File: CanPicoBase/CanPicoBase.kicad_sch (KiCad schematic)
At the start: 17 parts, among them J1 3.50 CBUS, J2 5V select, J3 Grove 2mm, J4 Conn_01x20_Male, J5 Conn_01x20_Male, Q1 DMG2305UX-7, U1 AMS1117-5.0, U2 AMS1117-3.3, U3 Pico

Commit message: 20:38 Arrakis.local
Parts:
- J4, J5: footprint Connector_PinHeader_2.54mm:PinHeader_1x20_P2.54mm_Vertical -> Connector_PinSocket_2.54mm:PinSocket_1x20_P2.54mm_Vertical
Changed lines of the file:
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@@
     (property "Reference" "J4" (id 0) (at 191.135 34.29 0))
     (property "Value" "Conn_01x20_Male" (id 1) (at 191.135 36.83 0))
-    (property "Footprint" "Connector_PinHeader_2.54mm:PinHeader_1x20_P2.54mm_Vertical" (id 2) (at 190.5 62.23 0)
+    (property "Footprint" "Connector_PinSocket_2.54mm:PinSocket_1x20_P2.54mm_Vertical" (id 2) (at 190.5 62.23 0)
       (effects (font (size 1.27 1.27)) hide)
     )
@@
       (effects (font (size 1.27 1.27)) (justify right))
     )
-    (property "Footprint" "Connector_PinHeader_2.54mm:PinHeader_1x20_P2.54mm_Vertical" (id 2) (at 273.05 64.77 0)
+    (property "Footprint" "Connector_PinSocket_2.54mm:PinSocket_1x20_P2.54mm_Vertical" (id 2) (at 273.05 64.77 0)
       (effects (font (size 1.27 1.27)) hide)
     )
@@
     )
     (path "/1a850953-e696-40b6-a1fc-7a92a62063d4"
-      (reference "J4") (unit 1) (value "Conn_01x20_Male") (footprint "Connector_PinHeader_2.54mm:PinHeader_1x20_P2.54mm_Vertical")
+      (reference "J4") (unit 1) (value "Conn_01x20_Male") (footprint "Connector_PinSocket_2.54mm:PinSocket_1x20_P2.54mm_Vertical")
     )
     (path "/508c1793-b3ac-4a28-93d9-e73559a97305"
-      (reference "J5") (unit 1) (value "Conn_01x20_Male") (footprint "Connector_PinHeader_2.54mm:PinHeader_1x20_P2.54mm_Vertical")
+      (reference "J5") (unit 1) (value "Conn_01x20_Male") (footprint "Connector_PinSocket_2.54mm:PinSocket_1x20_P2.54mm_Vertical")
     )
     (path "/37118974-3a56-4fcc-9031-fa4d14c74939"

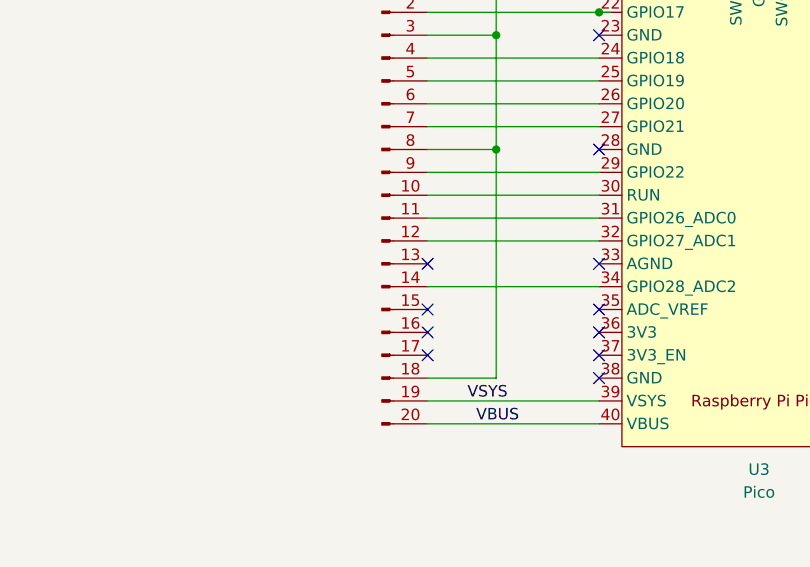
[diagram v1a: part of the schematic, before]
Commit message: 21:37 Titan.local
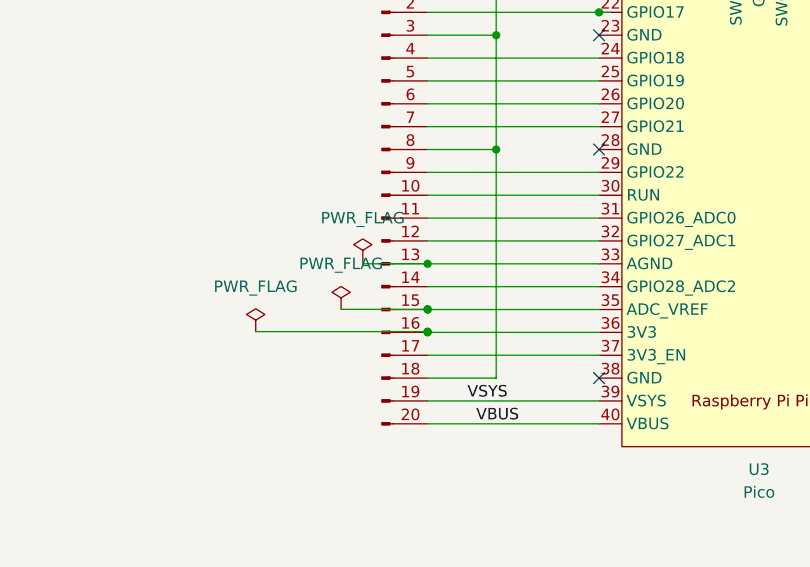
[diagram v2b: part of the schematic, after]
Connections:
- net at J4.13 (Pin_13): now also U3.33 (AGND)
- net at J4.15 (Pin_15): now also U3.35 (ADC_VREF)
- net at J4.16 (Pin_16): now also U3.36 (3V3)
- net at J4.17 (Pin_17): now also U3.37 (3V3_EN)
- no-connect marks 19 -> 11
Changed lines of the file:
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@@
   (junction (at 267.97 82.55) (diameter 0) (color 0 0 0 0)
   )
+  (junction (at 195.58 77.3836) (diameter 0) (color 0 0 0 0)
+  )
   (junction (at 34.065 120.5719) (diameter 0) (color 0 0 0 0)
   )
+  (junction (at 195.58 74.9115) (diameter 0) (color 0 0 0 0)
+  )
   (junction (at 58.42 62.1444) (diameter 0) (color 0 0 0 0)
   )
@@
   (junction (at 214.63 41.91) (diameter 0) (color 0 0 0 0)
   )
+  (junction (at 195.58 74.93) (diameter 0) (color 0 0 0 0)
+  )
   (junction (at 257.81 57.15) (diameter 0) (color 0 0 0 0)
   )
@@
   (junction (at 57.15 100.2425) (diameter 0) (color 0 0 0 0)
   )
+  (junction (at 195.58 77.47) (diameter 0) (color 0 0 0 0)
+  )
   (junction (at 203.2 44.45) (diameter 0) (color 0 0 0 0)
   )
+  (junction (at 195.58 69.85) (diameter 0) (color 0 0 0 0)
+  )
   (no_connect (at 250.19 69.85))
-  (no_connect (at 214.63 80.01))
-  (no_connect (at 195.58 69.85))
   (no_connect (at 214.63 82.55))
-  (no_connect (at 195.58 80.01))
   (no_connect (at 234.95 34.29))
   (no_connect (at 250.19 57.15))
@@
   (no_connect (at 22.86 29.21))
   (no_connect (at 229.87 34.29))
-  (no_connect (at 214.63 77.47))
-  (no_connect (at 195.58 74.93))
-  (no_connect (at 214.63 69.85))
   (no_connect (at 214.63 44.45))
-  (no_connect (at 214.63 74.93))
-  (no_connect (at 195.58 77.47))
   (no_connect (at 214.63 57.15))
   (wire (pts (xy 250.19 82.55) (xy 257.81 82.55))
@@
     (stroke (width 0) (type default) (color 0 0 0 0))
   )
+  (wire (pts (xy 188.379 69.85) (xy 195.58 69.85))
+    (stroke (width 0) (type default) (color 0 0 0 0))
+  )
   (wire (pts (xy 58.42 48.26) (xy 58.42 52.07))
     (stroke (width 0) (type default) (color 0 0 0 0))
@@
     (stroke (width 0) (type default) (color 0 0 0 0))
   )
+  (wire (pts (xy 195.58 77.3836) (xy 195.58 77.47))
+    (stroke (width 0) (type default) (color 0 0 0 0))
+  )
   (wire (pts (xy 250.19 41.91) (xy 267.97 41.91))
     (stroke (width 0) (type default) (color 0 0 0 0))
@@
     (stroke (width 0) (type default) (color 0 0 0 0))
   )
+  (wire (pts (xy 185.9652 74.9115) (xy 195.58 74.9115))
+    (stroke (width 0) (type default) (color 0 0 0 0))
+  )
   (wire (pts (xy 203.2 44.45) (xy 203.2 57.15))
     (stroke (width 0) (type default) (color 0 0 0 0))
@@
     (stroke (width 0) (type default) (color 0 0 0 0))
   )
+  (wire (pts (xy 195.58 74.93) (xy 214.63 74.93))
+    (stroke (width 0) (type default) (color 0 0 0 0))
+  )
   (wire (pts (xy 83.82 33.02) (xy 83.82 48.26))
     (stroke (width 0) (type default) (color 0 0 0 0))
@@
     (stroke (width 0) (type default) (color 0 0 0 0))
   )
+  (wire (pts (xy 176.4825 77.3828) (xy 195.58 77.3836))
+    (stroke (width 0) (type default) (color 0 0 0 0))
+  )
   (wire (pts (xy 29.21 120.65) (xy 34.065 120.65))
     (stroke (width 0) (type default) (color 0 0 0 0))
@@
     (stroke (width 0) (type default) (color 0 0 0 0))
   )
+  (wire (pts (xy 195.58 74.9115) (xy 195.58 74.93))
+    (stroke (width 0) (type default) (color 0 0 0 0))
+  )
   (wire (pts (xy 195.58 59.69) (xy 214.63 59.69))
     (stroke (width 0) (type default) (color 0 0 0 0))
@@
     (stroke (width 0) (type default) (color 0 0 0 0))
   )
+  (wire (pts (xy 195.58 77.47) (xy 214.63 77.47))
+    (stroke (width 0) (type default) (color 0 0 0 0))
+  )
   (wire (pts (xy 250.19 46.99) (xy 267.97 46.99))
     (stroke (width 0) (type default) (color 0 0 0 0))
@@
     (stroke (width 0) (type default) (color 0 0 0 0))
   )
+  (wire (pts (xy 195.58 80.01) (xy 214.63 80.01))
+    (stroke (width 0) (type default) (color 0 0 0 0))
+  )
   (wire (pts (xy 69.5486 180.6696) (xy 69.5486 180.8186))
+    (stroke (width 0) (type default) (color 0 0 0 0))
+  )
+  (wire (pts (xy 188.379 69.85) (xy 188.379 69.6241))
+    (stroke (width 0) (type default) (color 0 0 0 0))
+  )
+  (wire (pts (xy 195.58 69.85) (xy 214.63 69.85))
     (stroke (width 0) (type default) (color 0 0 0 0))
   )
@@
     (pin "1")
   )
+  (symbol (lib_id "power:PWR_FLAG") (at 185.9652 74.9115 0) (unit 1)
+    (in_bom yes) (on_board yes) (fields_autoplaced)
+    (property "Reference" "#FLG05" (id 0) (at 185.9652 73.0065 0)
+      (effects (font (size 1.27 1.27)) hide)
+    )
+    (property "Value" "PWR_FLAG" (id 1) (at 185.9652 69.85 0))
+    (property "Footprint" "" (id 2) (at 185.9652 74.9115 0)
+      (effects (font (size 1.27 1.27)) hide)
+    )
+    (property "Datasheet" "~" (id 3) (at 185.9652 74.9115 0)
+      (effects (font (size 1.27 1.27)) hide)
+    )
+    (pin "1")
+  )
   (symbol (lib_id "power:PWR_FLAG") (at 102.87 43.18 0) (unit 1)
     (in_bom yes) (on_board yes) (fields_autoplaced)
@@
     (pin "4")
   )
+  (symbol (lib_id "power:PWR_FLAG") (at 176.4825 77.3828 0) (unit 1)
+    (in_bom yes) (on_board yes) (fields_autoplaced)
+    (property "Reference" "#FLG02" (id 0) (at 176.4825 75.4778 0)
+      (effects (font (size 1.27 1.27)) hide)
+    )
+    (property "Value" "PWR_FLAG" (id 1) (at 176.4825 72.3892 0))
+    (property "Footprint" "" (id 2) (at 176.4825 77.3828 0)
+      (effects (font (size 1.27 1.27)) hide)
+    )
+    (property "Datasheet" "~" (id 3) (at 176.4825 77.3828 0)
+      (effects (font (size 1.27 1.27)) hide)
+    )
+    (pin "1")
+  )
   (symbol (lib_id "Connector:Screw_Terminal_01x04") (at 17.78 26.67 0) (mirror y) (unit 1)
     (in_bom yes) (on_board yes)
@@
     )
     (property "Datasheet" "" (id 3) (at 27.4135 31.9563 0)
+      (effects (font (size 1.27 1.27)) hide)
+    )
+    (pin "1")
+  )
+  (symbol (lib_id "power:PWR_FLAG") (at 188.379 69.6241 0) (unit 1)
+    (in_bom yes) (on_board yes) (fields_autoplaced)
+    (property "Reference" "#FLG07" (id 0) (at 188.379 67.7191 0)
+      (effects (font (size 1.27 1.27)) hide)
+    )
+    (property "Value" "PWR_FLAG" (id 1) (at 188.379 64.77 0))
+    (property "Footprint" "" (id 2) (at 188.379 69.6241 0)
+      (effects (font (size 1.27 1.27)) hide)
+    )
+    (property "Datasheet" "~" (id 3) (at 188.379 69.6241 0)
       (effects (font (size 1.27 1.27)) hide)
     )
@@
       (reference "#FLG01") (unit 1) (value "PWR_FLAG") (footprint "")
     )
+    (path "/576b0112-b207-4bf3-8c1d-a5c23dcda14e"
+      (reference "#FLG02") (unit 1) (value "PWR_FLAG") (footprint "")
+    )
     (path "/29410c01-763d-4c52-8a72-4db199a9dfe7"
       (reference "#FLG03") (unit 1) (value "PWR_FLAG") (footprint "")
@@
       (reference "#FLG04") (unit 1) (value "PWR_FLAG") (footprint "")
     )
+    (path "/2112fe59-d187-4c42-afed-65235cd0d021"
+      (reference "#FLG05") (unit 1) (value "PWR_FLAG") (footprint "")
+    )
     (path "/25d52506-8d92-4dfa-bd69-530ed70b2860"
       (reference "#FLG06") (unit 1) (value "PWR_FLAG") (footprint "")
     )
+    (path "/97181b30-8464-4d71-943e-45f9bae00245"
+      (reference "#FLG07") (unit 1) (value "PWR_FLAG") (footprint "")
+    )
     (path "/95f09844-5459-48d5-92f4-372322dbe922"
